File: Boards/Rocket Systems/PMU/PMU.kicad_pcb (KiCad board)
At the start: 4 copper layers, 152 x 71 mm, 146 parts, among them IC1 LM4040DIZ-4.1_NOPB, IC2 LM4040DIZ-4.1_NOPB, IC3 LM4040DIZ-4.1_NOPB, IC4 LS1205EFD33, J1 172298-1104, J10 1723163304, J2 XT30UPB-F, J3 XT30UPB-F, J4 XT30UPB-F, J5 XT30UPB-F, J6 1723163304, J8 XT30UPB-F, J9 1723163304, K3 G3VM-31DR_TR05_, K4 G3VM-31DR_TR05_, K5 G3VM-31DR_TR05_, Q1 NPN, Q2 PMOS, Q3 NPN, Q4 NPN, Q5 NPN, Q6 NPN, Q7 NPN, Q8 NPN, U10 ST1L05APU33R, U11 NCR321UX, U12 NCR321UX, U13 NCR321UX, U29 NCV8114ASN165T1G, U3 STPS15L45CB, U30 MCP6002-E/MS, U4 STPS15L45CB, U7 NJD35N04T4G, U8 NJD35N04T4G, U9 NJD35N04T4G

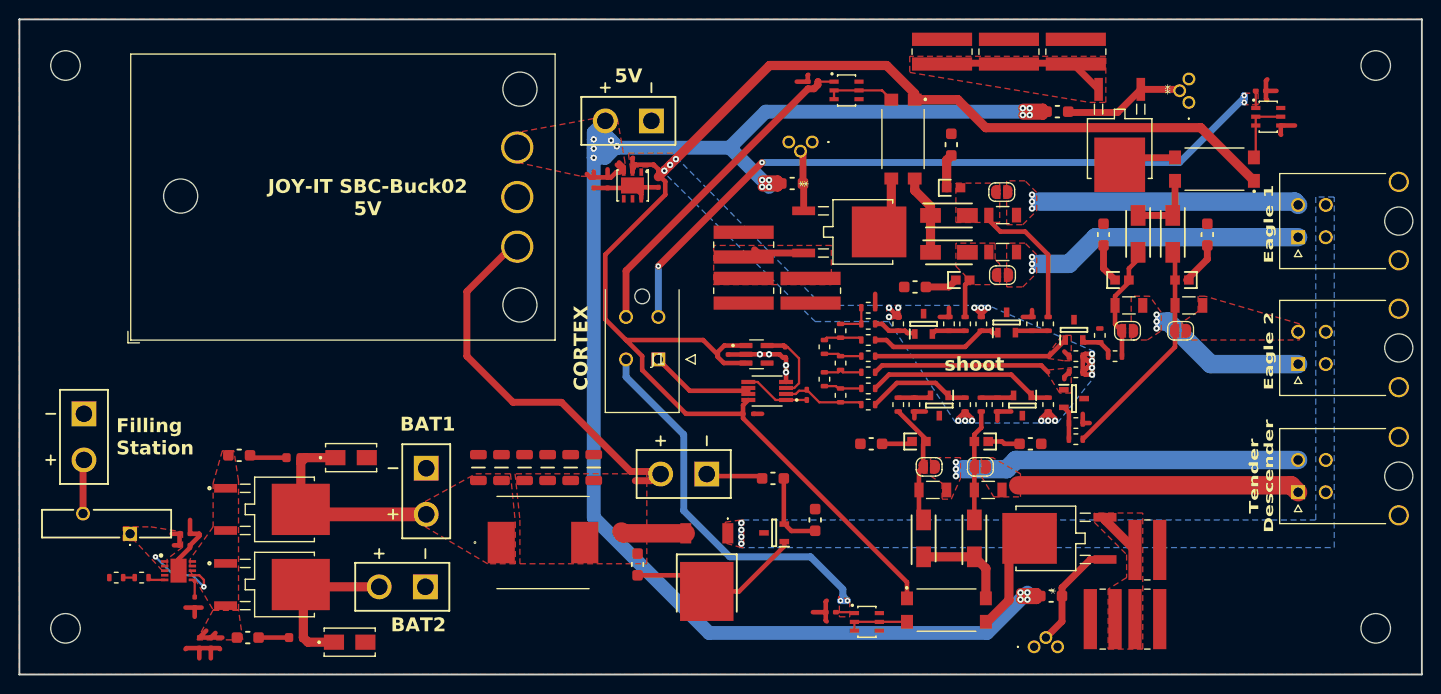
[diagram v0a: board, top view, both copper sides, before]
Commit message: PMU banger
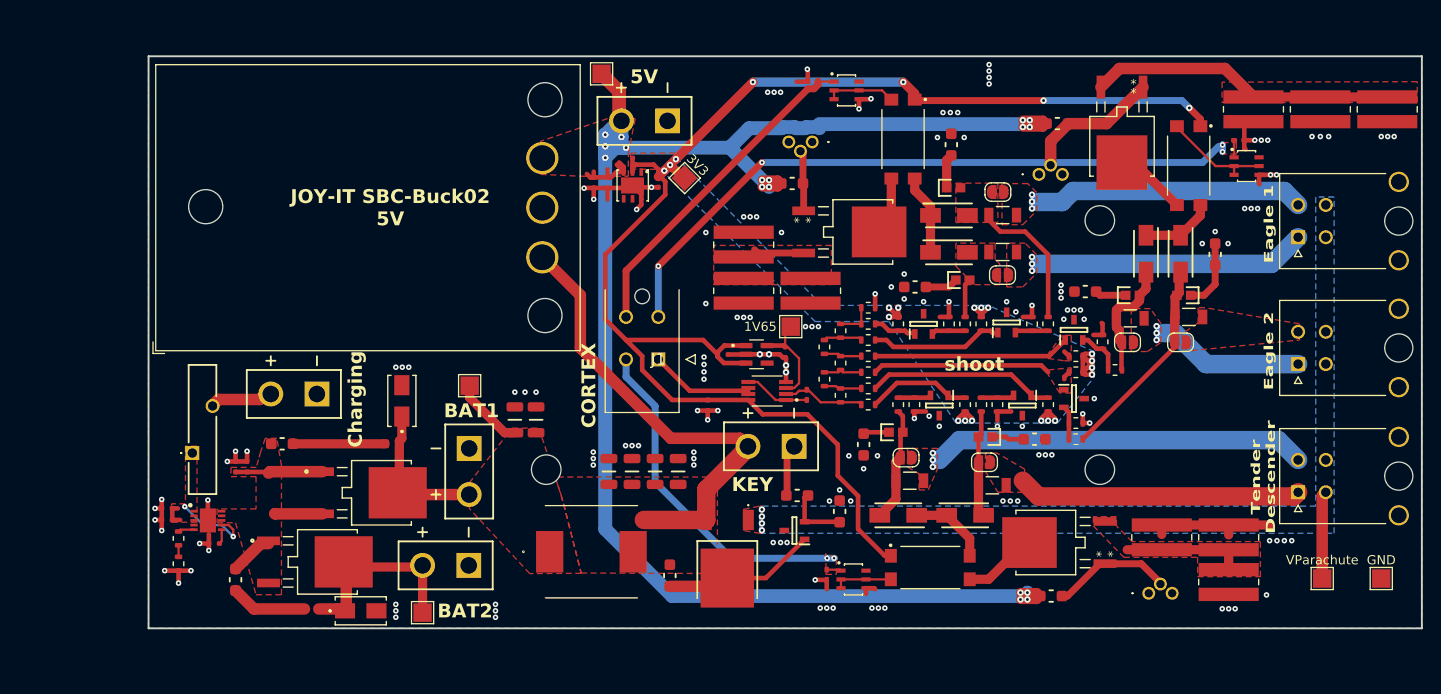
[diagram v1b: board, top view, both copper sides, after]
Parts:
- removed the H2 at (82.5, 46.0)
- removed the H2 at (224.5, 107.0)
- removed the H2 at (224.5, 46.0)
- removed the H2 at (82.5, 107.0)
- added 1V65: TestPoint, TestPoint:TestPoint_Pad_2.0x2.0mm, F.Cu at (161.1, 74.3)
- added 3V3: TestPoint, TestPoint:TestPoint_Pad_2.0x2.0mm, F.Cu at (149.6, 58.2)
- added 5V: TestPoint, TestPoint:TestPoint_Pad_2.0x2.0mm, F.Cu at (140.6, 46.9)
- added GND: TestPoint, TestPoint:TestPoint_Pad_2.0x2.0mm, F.Cu at (225.1, 101.6)
- added H1: MountingHole, MountingHole:MountingHole_3.2mm_M3_ISO7380, F.Cu at (194.6, 89.8)
- added H2: MountingHole, MountingHole:MountingHole_3.2mm_M3_ISO7380, F.Cu at (194.6, 62.8)
- added H3: MountingHole, MountingHole:MountingHole_3.2mm_M3_ISO7380, F.Cu at (134.6, 89.8)
- added VBAT1: TestPoint, TestPoint:TestPoint_Pad_2.0x2.0mm, F.Cu at (126.3, 80.7)
- added VBAT2: TestPoint, TestPoint:TestPoint_Pad_2.0x2.0mm, F.Cu at (121.2, 105.3)
- added VParachute: TestPoint, TestPoint:TestPoint_Pad_2.0x2.0mm, F.Cu at (218.7, 101.6)
- moved R26 48.7 mm to (225.8, 50.8), turned to -90 degrees
- moved R25 34.3 mm to (218.5, 50.8), turned to -90 degrees
- moved J4 25.3 mm to (109.8, 81.6), turned to 90 degrees
- moved R24 20.2 mm to (211.2, 50.8), turned to -90 degrees
- moved C41 19.8 mm to (102.2, 89.5), turned to -90 degrees
- moved C42 19.3 mm to (100.9, 89.5), turned to -90 degrees
- moved IC2 18.0 mm to (188.0, 57.8), turned to 0 degrees
- moved R29 14.2 mm to (208.6, 102.0), turned to -90 degrees
- moved IC3 13.7 mm to (199.9, 103.2)
- moved R30 12.5 mm to (208.6, 97.1), turned to 90 degrees
- moved F7 11.1 mm to (96.2, 88.0), turned to 90 degrees
- moved C9 10.8 mm to (117.9, 87.0)
- moved U3 10.7 mm to (116.7, 92.3)
- moved J5 9.93 mm to (161.5, 87.3)
- moved C3 9.16 mm to (141.4, 90.0)
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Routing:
- net GND: track 58.5 -> 90.5 mm, vias 4 -> 148
- net Net-(U8-E): track 16.6 -> 33.2 mm
- net Net-(IC4-OUT_1): track 4.27 -> 19.4 mm
- net +3.3V: track 192.6 -> 182.9 mm, vias 19 -> 23
- net VParachute: track 0.00 -> 9.51 mm
- net Net-(U9-E): track 4.88 -> 13.2 mm
- net Net-(C9-Pad1): track 4.05 -> 10.3 mm
- net /RECOVERY3: track 44.6 -> 39.1 mm
- net Net-(C8-Pad2): track 3.30 -> 8.30 mm
- net /RECOVERY2: track 79.7 -> 74.7 mm
- net /FIRE_OUT2: track 7.20 -> 11.8 mm
- net VBAT2: track 18.0 -> 21.9 mm
- net /PYRO6_OUT: track 37.1 -> 40.6 mm
- net Net-(U8-C): track 6.33 -> 8.95 mm
- net +1.65V: track 8.35 -> 10.8 mm
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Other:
- board size 152 x 71 mm -> 138 x 62 mm
- board text added: "Charging"
- board text added: "KEY"
- board text removed: "Filling Station"
